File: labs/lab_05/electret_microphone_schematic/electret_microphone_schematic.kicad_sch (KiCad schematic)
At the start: 9 parts, among them U1 TL081, U2 TL081

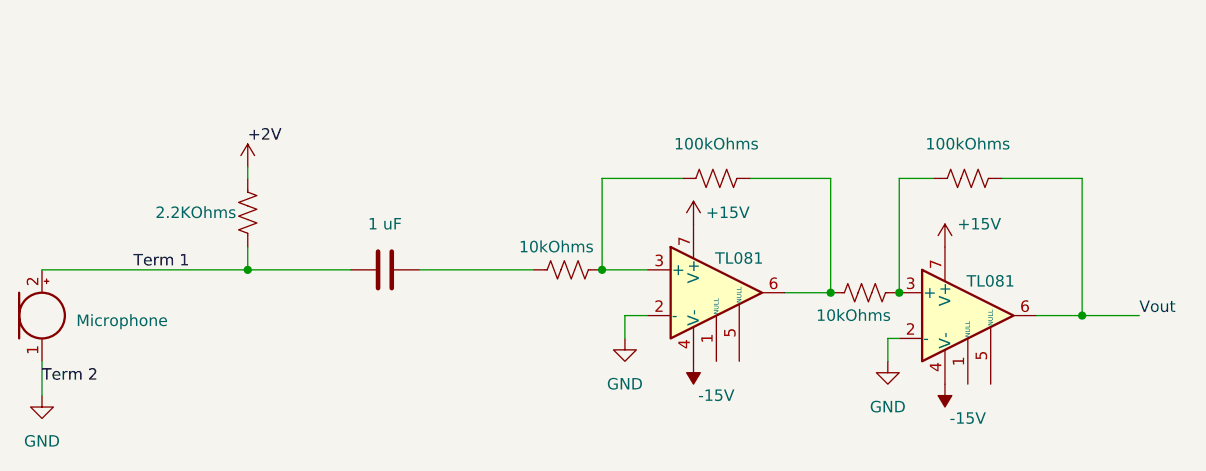
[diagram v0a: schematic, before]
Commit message: edits? acoustics
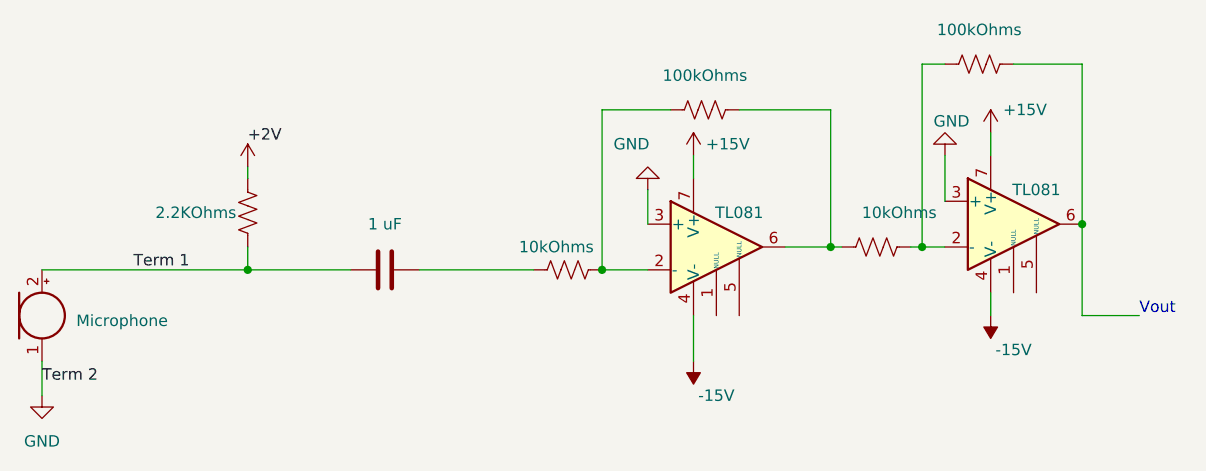
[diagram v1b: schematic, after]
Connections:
- net GND: now also U1.3 (+), U2.3 (+); no longer U1.2 (-), U2.2 (-)
- net at R3.2, R4.1: now also U2.2 (-); no longer U2.3 (+)
- net at R1.2, R2.1: now also U1.2 (-); no longer U1.3 (+)
